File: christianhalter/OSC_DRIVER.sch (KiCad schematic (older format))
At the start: 6 parts, among them U1 SN74LVC1GX04

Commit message: Gerber
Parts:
- C1, C2, C3: footprint halter:C_0805_HandSoldering -> halter:C_0603_HandSoldering
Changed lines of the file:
@@
 F 0 "C3" H 7100 2350 60  0000 C CNN
 F 1 "100nF" H 7200 2050 60  0000 R CNN
-F 2 "halter:C_0805_HandSoldering" H 7100 2200 60  0001 C CNN
+F 2 "halter:C_0603_HandSoldering" H 7100 2200 60  0001 C CNN
 F 3 "" H 7100 2200 60  0000 C CNN
 F 4 "Value" H 7100 2200 60  0001 C CNN "Digikey/Mouser"
@@
 F 0 "C1" H 5100 4050 60  0000 C CNN
 F 1 "33pF" H 5200 3750 60  0000 R CNN
-F 2 "halter:C_0805_HandSoldering" H 5100 3900 60  0001 C CNN
+F 2 "halter:C_0603_HandSoldering" H 5100 3900 60  0001 C CNN
 F 3 "" H 5100 3900 60  0000 C CNN
 F 4 "Value" H 5100 3900 60  0001 C CNN "Digikey/Mouser"
@@
 F 0 "C2" H 6100 4050 60  0000 C CNN
 F 1 "33pF" H 6200 3750 60  0000 R CNN
-F 2 "halter:C_0805_HandSoldering" H 6100 3900 60  0001 C CNN
+F 2 "halter:C_0603_HandSoldering" H 6100 3900 60  0001 C CNN
 F 3 "" H 6100 3900 60  0000 C CNN
 F 4 "Value" H 6100 3900 60  0001 C CNN "Digikey/Mouser"

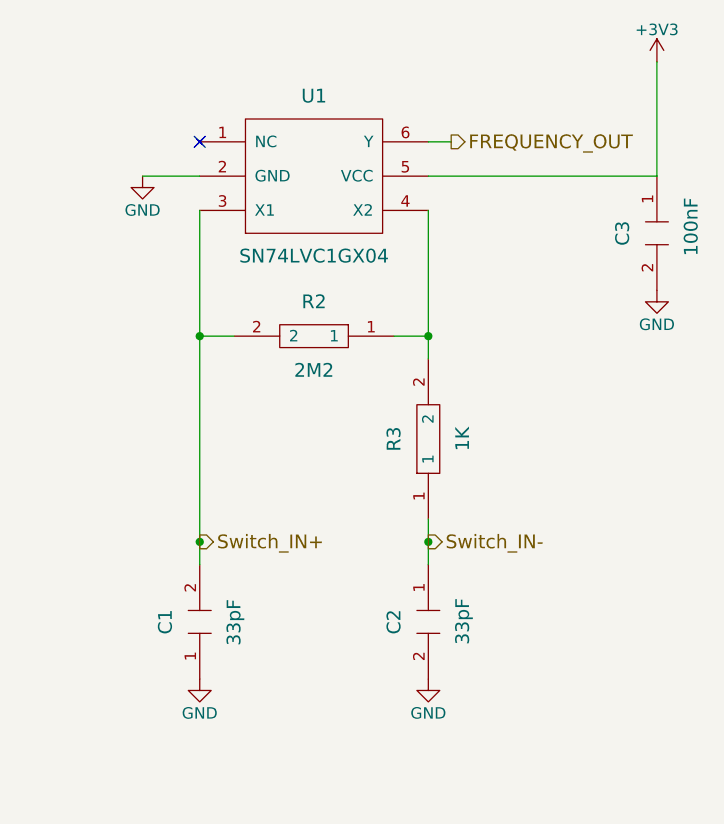
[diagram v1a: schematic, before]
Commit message: Libreria nueva
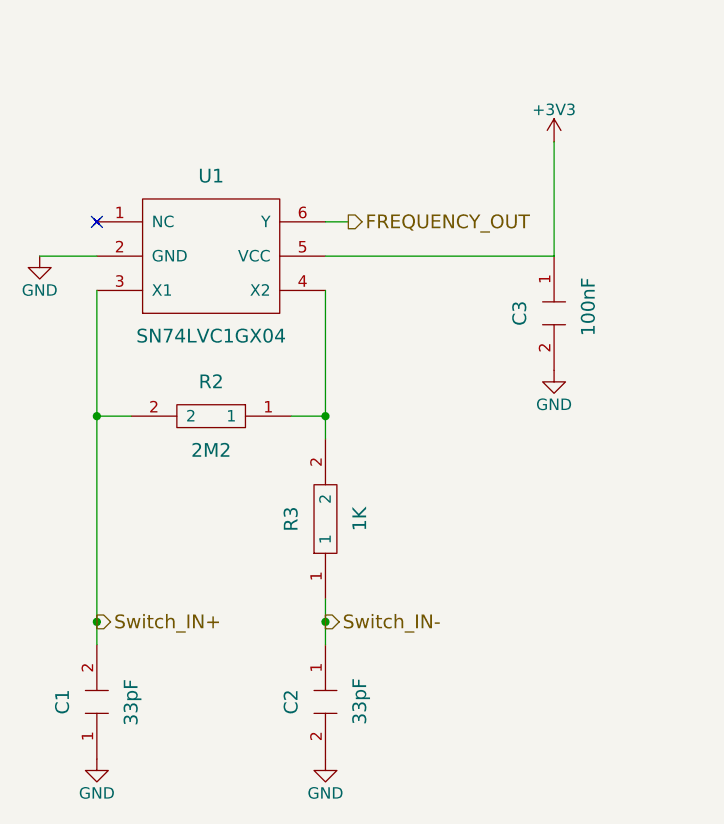
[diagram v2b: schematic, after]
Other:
- moved on the sheet: C1, C2, C3, R2, R3, U1
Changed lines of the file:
@@
 LIBS:XTAL_SMD_HandSoldering
 LIBS:ltc5507
+LIBS:74hct4053_pringle
 LIBS:halter-cache
 EELAYER 25 0
@@
 L SN74LVC1GX04 U1
 U 1 1 56E7582E
-P 5600 1950
-F 0 "U1" H 5600 2300 60  0000 C CNN
-F 1 "SN74LVC1GX04" H 5600 1600 60  0000 C CNN
-F 2 "halter:SOT-23-6" H 5600 1950 60  0001 C CNN
-F 3 "" H 5600 1950 60  0000 C CNN
-F 4 "Value" H 5600 1950 60  0001 C CNN "Digikey/Mouser"
-	1    5600 1950
+P 5150 2300
+F 0 "U1" H 5150 2650 60  0000 C CNN
+F 1 "SN74LVC1GX04" H 5150 1950 60  0000 C CNN
+F 2 "halter:SOT-23-6" H 5150 2300 60  0001 C CNN
+F 3 "" H 5150 2300 60  0000 C CNN
+F 4 "Value" H 5150 2300 60  0001 C CNN "Digikey/Mouser"
+	1    5150 2300
 	1    0    0    -1
 $EndComp
@@
 L +3V3 #PWR010
 U 1 1 56E75836
-P 7100 1450
-F 0 "#PWR010" H 7100 1300 50  0001 C CNN
-F 1 "+3V3" H 7100 1590 50  0000 C CNN
-F 2 "" H 7100 1450 60  0000 C CNN
-F 3 "" H 7100 1450 60  0000 C CNN
-	1    7100 1450
+P 6650 1800
+F 0 "#PWR010" H 6650 1650 50  0001 C CNN
+F 1 "+3V3" H 6650 1940 50  0000 C CNN
+F 2 "" H 6650 1800 60  0000 C CNN
+F 3 "" H 6650 1800 60  0000 C CNN
+	1    6650 1800
 	1    0    0    -1
 $EndComp
 Wire Wire Line
-	6100 1800 6200 1800
+	5650 2150 5750 2150
 Wire Wire Line
-	6100 1950 7100 1950
+	5650 2300 6650 2300
 Wire Wire Line
-	7100 1950 7100 1450
-NoConn ~ 5100 1800
+	6650 2300 6650 1800
+NoConn ~ 4650 2150
 $Comp
 L GND #PWR011
 U 1 1 56E75840
-P 4850 1950
-F 0 "#PWR011" H 4850 1700 50  0001 C CNN
-F 1 "GND" H 4850 1800 50  0000 C CNN
-F 2 "" H 4850 1950 60  0000 C CNN
-F 3 "" H 4850 1950 60  0000 C CNN
-	1    4850 1950
+P 4400 2300
+F 0 "#PWR011" H 4400 2050 50  0001 C CNN
+F 1 "GND" H 4400 2150 50  0000 C CNN
+F 2 "" H 4400 2300 60  0000 C CNN
+F 3 "" H 4400 2300 60  0000 C CNN
+	1    4400 2300
 	1    0    0    -1
 $EndComp
 Wire Wire Line
-	5100 1950 4850 1950
+	4650 2300 4400 2300
 $Comp
 L Capacitor_SMD_HandSoldering C3
 U 1 1 56E75848
-P 7100 2200
-F 0 "C3" H 7100 2350 60  0000 C CNN
-F 1 "100nF" H 7200 2050 60  0000 R CNN
-F 2 "halter:C_0603_HandSoldering" H 7100 2200 60  0001 C CNN
-F 3 "" H 7100 2200 60  0000 C CNN
-F 4 "Value" H 7100 2200 60  0001 C CNN "Digikey/Mouser"
-	1    7100 2200
+P 6650 2550
+F 0 "C3" H 6650 2700 60  0000 C CNN
+F 1 "100nF" H 6750 2400 60  0000 R CNN
+F 2 "halter:C_0603_HandSoldering" H 6650 2550 60  0001 C CNN
+F 3 "" H 6650 2550 60  0000 C CNN
+F 4 "Value" H 6650 2550 60  0001 C CNN "Digikey/Mouser"
+	1    6650 2550
 	0    -1   1    0
 $EndComp
@@
 L GND #PWR012
 U 1 1 56E7584F
-P 7100 2450
-F 0 "#PWR012" H 7100 2200 50  0001 C CNN
-F 1 "GND" H 7100 2300 50  0000 C CNN
-F 2 "" H 7100 2450 60  0000 C CNN
-F 3 "" H 7100 2450 60  0000 C CNN
-	1    7100 2450
+P 6650 2800
+F 0 "#PWR012" H 6650 2550 50  0001 C CNN
+F 1 "GND" H 6650 2650 50  0000 C CNN
+F 2 "" H 6650 2800 60  0000 C CNN
+F 3 "" H 6650 2800 60  0000 C CNN
+	1    6650 2800
 	1    0    0    -1
 $EndComp
 Wire Wire Line
-	7100 2450 7100 2450
+	6650 2800 6650 2800
 $Comp
 L Resistor_0805_HandSoldering R2
 U 1 1 56E75857
-P 5600 2650
-F 0 "R2" H 5600 2800 60  0000 C CNN
-F 1 "2M2" H 5600 2500 60  0000 C CNN
-F 2 "halter:R_0805_HandSoldering" H 5600 2650 60  0001 C CNN
-F 3 "" H 5600 2650 60  0000 C CNN
-F 4 "Value" H 5600 2650 60  0001 C CNN "Digikey/Mouser"
-	1    5600 2650
+P 5150 3000
+F 0 "R2" H 5150 3150 60  0000 C CNN
+F 1 "2M2" H 5150 2850 60  0000 C CNN
+F 2 "halter:R_0805_HandSoldering" H 5150 3000 60  0001 C CNN
+F 3 "" H 5150 3000 60  0000 C CNN
+F 4 "Value" H 5150 3000 60  0001 C CNN "Digikey/Mouser"
+	1    5150 3000
 	-1   0    0    -1
 $EndComp
@@
 L Resistor_0805_HandSoldering R3
 U 1 1 56E7585F
-P 6100 3100
-F 0 "R3" H 6100 3250 60  0000 C CNN
-F 1 "1K" H 6100 2950 60  0000 C CNN
-F 2 "halter:R_0805_HandSoldering" H 6100 3100 60  0001 C CNN
-F 3 "" H 6100 3100 60  0000 C CNN
-F 4 "Value" H 6100 3100 60  0001 C CNN "Digikey/Mouser"
-	1    6100 3100
+P 5650 3450
+F 0 "R3" H 5650 3600 60  0000 C CNN
+F 1 "1K" H 5650 3300 60  0000 C CNN
+F 2 "halter:R_0805_HandSoldering" H 5650 3450 60  0001 C CNN
+F 3 "" H 5650 3450 60  0000 C CNN
+F 4 "Value" H 5650 3450 60  0001 C CNN "Digikey/Mouser"
+	1    5650 3450
 	0    -1   -1   0
 $EndComp
@@
 L Capacitor_SMD_HandSoldering C1
 U 1 1 56E75867
-P 5100 3900
-F 0 "C1" H 5100 4050 60  0000 C CNN
-F 1 "33pF" H 5200 3750 60  0000 R CNN
-F 2 "halter:C_0603_HandSoldering" H 5100 3900 60  0001 C CNN
-F 3 "" H 5100 3900 60  0000 C CNN
-F 4 "Value" H 5100 3900 60  0001 C CNN "Digikey/Mouser"
-	1    5100 3900
+P 4650 4250
+F 0 "C1" H 4650 4400 60  0000 C CNN
+F 1 "33pF" H 4750 4100 60  0000 R CNN
+F 2 "halter:C_0603_HandSoldering" H 4650 4250 60  0001 C CNN
+F 3 "" H 4650 4250 60  0000 C CNN
+F 4 "Value" H 4650 4250 60  0001 C CNN "Digikey/Mouser"
+	1    4650 4250
 	0    -1   -1   0
 $EndComp
@@
 L Capacitor_SMD_HandSoldering C2
 U 1 1 56E7586F
-P 6100 3900
-F 0 "C2" H 6100 4050 60  0000 C CNN
-F 1 "33pF" H 6200 3750 60  0000 R CNN
-F 2 "halter:C_0603_HandSoldering" H 6100 3900 60  0001 C CNN
-F 3 "" H 6100 3900 60  0000 C CNN
-F 4 "Value" H 6100 3900 60  0001 C CNN "Digikey/Mouser"
-	1    6100 3900
+P 5650 4250
+F 0 "C2" H 5650 4400 60  0000 C CNN
+F 1 "33pF" H 5750 4100 60  0000 R CNN
+F 2 "halter:C_0603_HandSoldering" H 5650 4250 60  0001 C CNN
+F 3 "" H 5650 4250 60  0000 C CNN
+F 4 "Value" H 5650 4250 60  0001 C CNN "Digikey/Mouser"
+	1    5650 4250
 	0    -1   1    0
 $EndComp
@@
 L GND #PWR013
 U 1 1 56E75876
-P 5100 4150
-F 0 "#PWR013" H 5100 3900 50  0001 C CNN
-F 1 "GND" H 5100 4000 50  0000 C CNN
-F 2 "" H 5100 4150 60  0000 C CNN
-F 3 "" H 5100 4150 60  0000 C CNN
-	1    5100 4150
+P 4650 4500
+F 0 "#PWR013" H 4650 4250 50  0001 C CNN
+F 1 "GND" H 4650 4350 50  0000 C CNN
+F 2 "" H 4650 4500 60  0000 C CNN
+F 3 "" H 4650 4500 60  0000 C CNN
+	1    4650 4500
 	1    0    0    -1
 $EndComp
@@
 L GND #PWR014
 U 1 1 56E7587C
-P 6100 4150
-F 0 "#PWR014" H 6100 3900 50  0001 C CNN
-F 1 "GND" H 6100 4000 50  0000 C CNN
-F 2 "" H 6100 4150 60  0000 C CNN
-F 3 "" H 6100 4150 60  0000 C CNN
-	1    6100 4150
+P 5650 4500
+F 0 "#PWR014" H 5650 4250 50  0001 C CNN
+F 1 "GND" H 5650 4350 50  0000 C CNN
+F 2 "" H 5650 4500 60  0000 C CNN
+F 3 "" H 5650 4500 60  0000 C CNN
+	1    5650 4500
 	1    0    0    -1
 $EndComp
 Wire Wire Line
-	5950 2650 6100 2650
+	5500 3000 5650 3000
 Wire Wire Line
-	6100 2100 6100 2750
-Connection ~ 6100 2650
+	5650 2450 5650 3100
+Connection ~ 5650 3000
 Wire Wire Line
-	5250 2650 5100 2650
+	4800 3000 4650 3000
 Wire Wire Line
-	5100 2100 5100 3650
+	4650 2450 4650 4000
 Wire Wire Line
-	6100 3450 6100 3650
-Connection ~ 5100 2650
-Connection ~ 6100 3550
-Connection ~ 5100 3550
-Text HLabel 5100 3550 2    60   Output ~ 0
+	5650 3800 5650 4000
+Connection ~ 4650 3000
+Connection ~ 5650 3900
+Connection ~ 4650 3900
+Text HLabel 4650 3900 2    60   Output ~ 0
 Switch_IN+
-Text HLabel 6100 3550 2    60   Output ~ 0
+Text HLabel 5650 3900 2    60   Output ~ 0
 Switch_IN-
-Text HLabel 6200 1800 2    60   Output ~ 0
+Text HLabel 5750 2150 2    60   Output ~ 0
 FREQUENCY_OUT
 $EndSCHEMATC
